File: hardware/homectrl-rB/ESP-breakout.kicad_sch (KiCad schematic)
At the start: 19 parts, among them J2 USB_C_Female_USB2_Small, SW1 SW_RESET, SW2 SW_BOOT, U1 ESP32-S3-WROOM-1

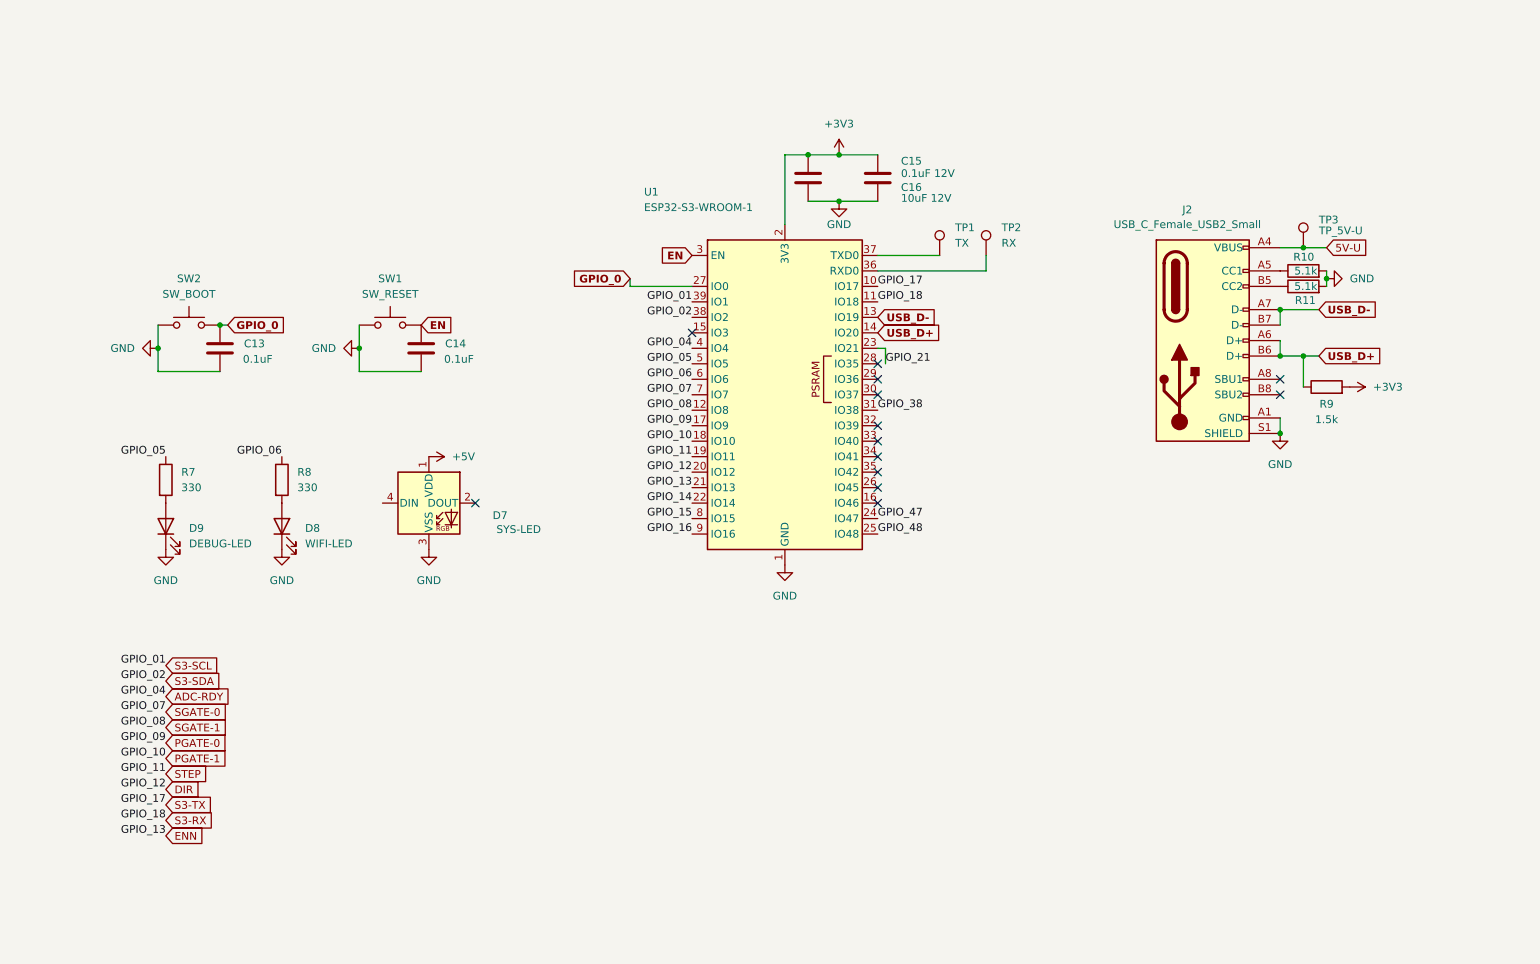
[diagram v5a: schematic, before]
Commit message: assign footprints
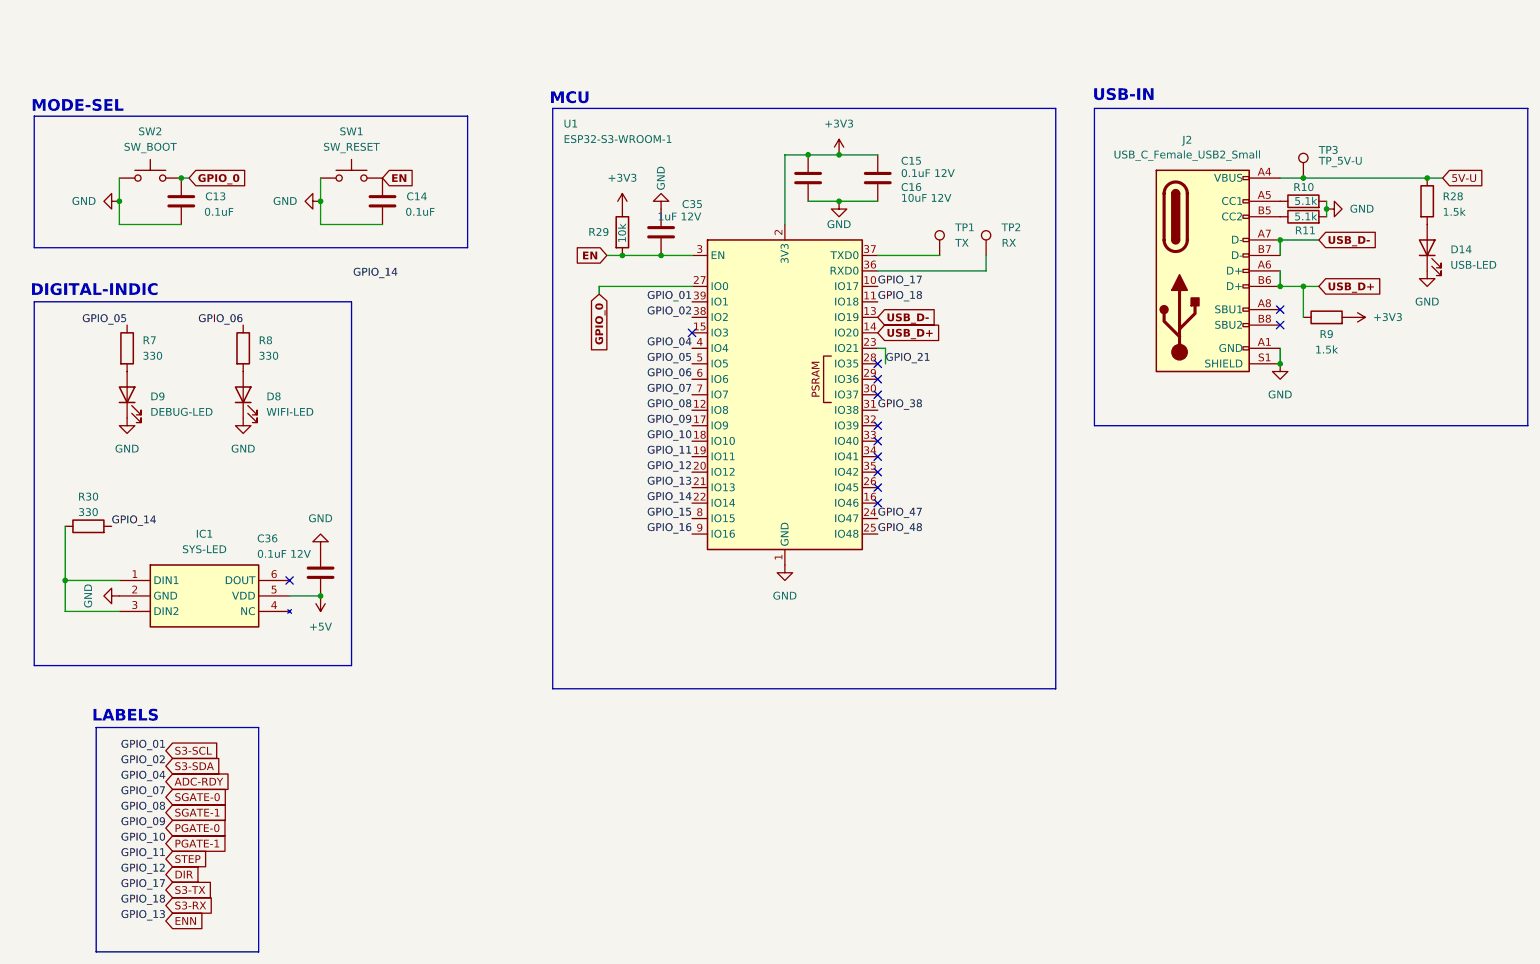
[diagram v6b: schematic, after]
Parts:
- removed D7: SYS-LED, LED_SMD:LED_WS2812B_PLCC4_5.0x5.0mm_P3.2mm, symbol LED:WS2812B
- added C35: 1uF 12V, Capacitor_SMD:C_0603_1608Metric, symbol Device:C
- added C36: 0.1uF 12V, Capacitor_SMD:C_0402_1005Metric, symbol Device:C
- added D14: USB-LED, LED_SMD:LED_0402_1005Metric, symbol Device:LED
- added IC1: SYS-LED, IN-PI20TBT5R5G5B:INPI20TBT5R5G5B, symbol IN-PI20TBT5R5G5B:IN-PI20TBT5R5G5B
- added R28: 1.5k, Resistor_SMD:R_0603_1608Metric, symbol Device:R
- added R29: 10k, Resistor_SMD:R_0402_1005Metric, symbol Device:R
- added R30: 330, Resistor_SMD:R_0402_1005Metric, symbol Device:R
- U1: footprint RF_Module:ESP32-S3-WROOM-1 -> ESP32-S3-WROOM-1-N16R2:XCVR_ESP32-S3-WROOM-1-N16R2
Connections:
- net +3V3: now also R29.1
- net +5V: now also C36.2, IC1.5 (VDD)
- net 5V-U: now also R28.1
- net EN: now also C35.1, R29.2
- net GND: now also C35.2, C36.1, D14.1 (K), IC1.2 (GND)
- net GPIO_14: now also R30.2
- new net: D14.2 (A), R28.2
- new net: IC1.1 (DIN1), IC1.3 (DIN2), R30.1
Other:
- note added: "DIGITAL-INDIC"
- note added: "LABELS"
- note added: "MCU"
- note added: "MODE-SEL"
- note added: "USB-IN"
- moved on the sheet: C13, C14, D8, D9, J2, R10, R11, R7, R8, R9, SW1, SW2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

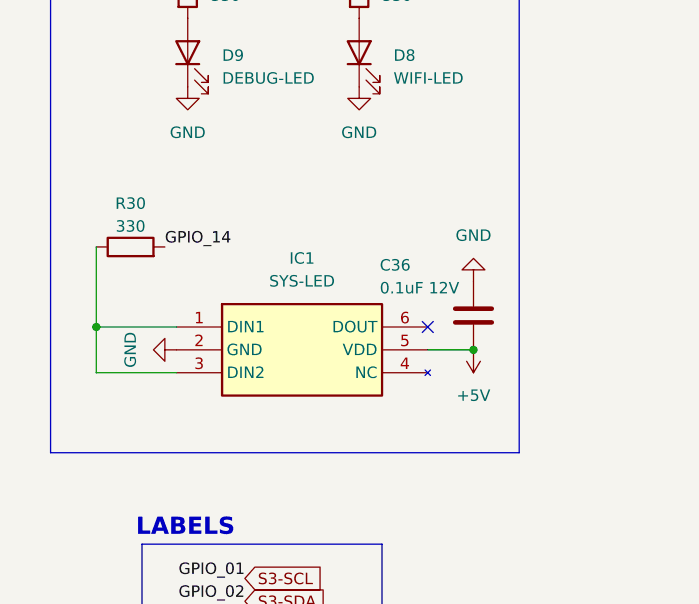
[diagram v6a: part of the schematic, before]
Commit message: layout work
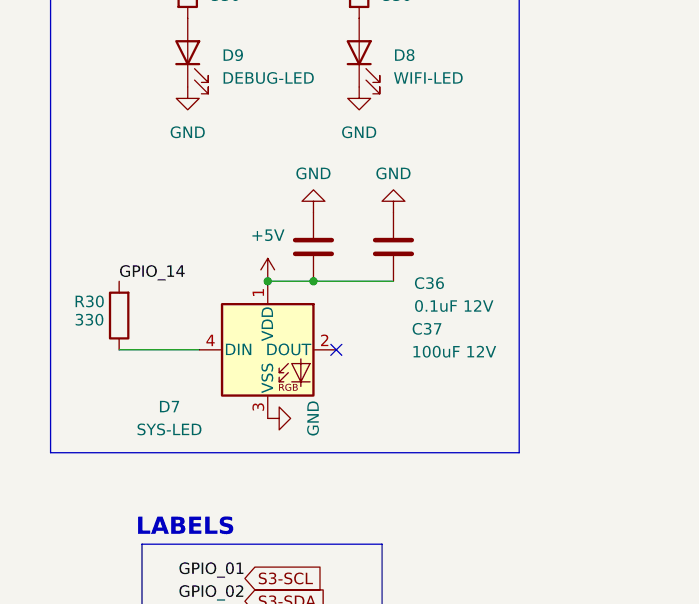
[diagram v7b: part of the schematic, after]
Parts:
- removed IC1: SYS-LED, IN-PI20TBT5R5G5B:INPI20TBT5R5G5B, symbol IN-PI20TBT5R5G5B:IN-PI20TBT5R5G5B
- added C37: 100uF 12V, Capacitor_SMD:C_1206_3216Metric, symbol Device:C
- added D7: SYS-LED, LED_SMD:LED_WS2812B_PLCC4_5.0x5.0mm_P3.2mm, symbol LED:WS2812B
- D14: footprint LED_SMD:LED_0402_1005Metric -> LED_SMD:LED_0603_1608Metric
- D8, D9: footprint Diode_SMD:D_0805_2012Metric -> LED_SMD:LED_0805_2012Metric
- R28: footprint Resistor_SMD:R_0603_1608Metric -> Resistor_SMD:R_0402_1005Metric
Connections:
- net +5V: now also C37.2, D7.1 (VDD)
- net GND: now also C37.1, D7.3 (VSS)
- net at R30.1: now also D7.4 (DIN)
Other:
- moved on the sheet: C36, R30

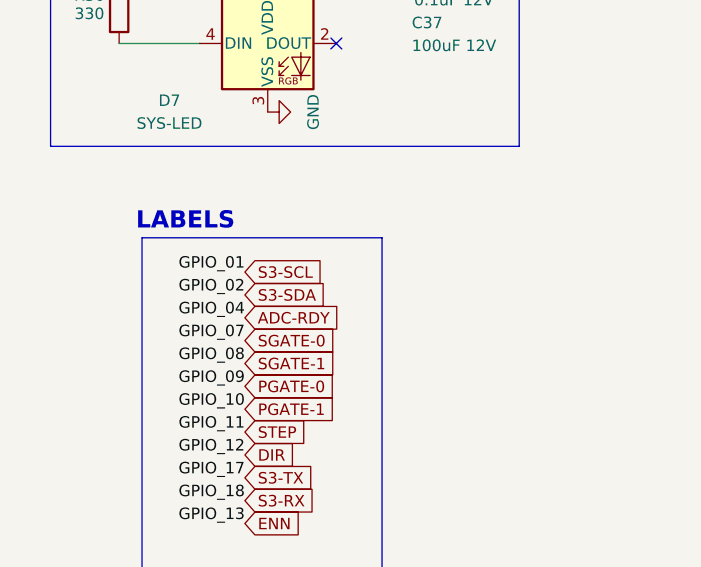
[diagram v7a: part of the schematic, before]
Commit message: routing work
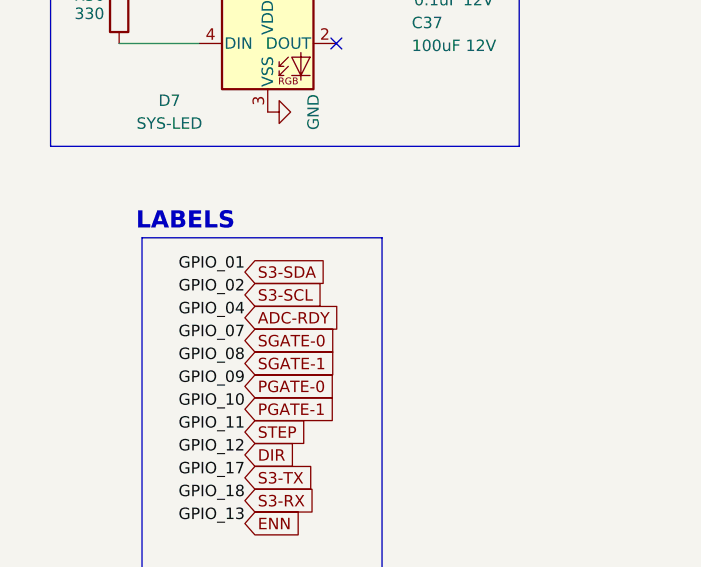
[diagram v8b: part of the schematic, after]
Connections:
- net S3-SCL: now also U1.38 (IO2); no longer U1.39 (IO1)
- net S3-SDA: now also U1.39 (IO1); no longer U1.38 (IO2)
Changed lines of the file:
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@@
+		)
+	)
+	(global_label "STEP"
+		(shape input)
+		(at 46.99 167.64 0)
+		(fields_autoplaced yes)
+		(effects
+			(font
+				(size 1.27 1.27)
+			)
+			(justify left)
+		)
+		(property "Intersheetrefs" "${INTERSHEET_REFS}"
+			(at 54.5713 167.64 0)
+			(effects
+				(font
+					(size 1.27 1.27)
+				)
+				(justify left)
+				(hide yes)
+			)
+		)
+	)
+	(global_label "ENN"
+		(shape input)
+		(at 46.99 177.8 0)
+		(fields_autoplaced yes)
+		(effects
+			(font
+				(size 1.27 1.27)
+			)
+			(justify left)
+		)
+		(property "Intersheetrefs" "${INTERSHEET_REFS}"
+			(at 53.7852 177.8 0)
+			(effects
+				(font
+					(size 1.27 1.27)
+				)
+				(justify left)
+				(hide yes)
+			)
+		)
+	)
+	(global_label "SGATE-1"
+		(shape input)
+		(at 46.99 160.02 0)
+		(fields_autoplaced yes)
+		(effects
+			(font
+				(size 1.27 1.27)
+			)
+			(justify left)
+		)
+		(property "Intersheetrefs" "${INTERSHEET_REFS}"
+			(at 58.4418 160.02 0)
+			(effects
+				(font
+					(size 1.27 1.27)
+				)
+				(justify left)
+				(hide yes)
+			)
+		)
+	)
+	(global_label "S3-SDA"
+		(shape input)
+		(at 46.99 149.86 0)
+		(fields_autoplaced yes)
+		(effects
+			(font
+				(size 1.27 1.27)
+			)
+			(justify left)
+		)
+		(property "Intersheetrefs" "${INTERSHEET_REFS}"
+			(at 57.5347 149.86 0)
+			(effects
+				(font
+					(size 1.27 1.27)
+				)
+				(justify left)
+				(hide yes)
+			)
 		)
 	)
 	(global_label "S3-SCL"
 		(shape input)
-		(at 46.99 149.86 0)
-		(fields_autoplaced yes)
-		(effects
-			(font
-				(size 1.27 1.27)
-			)
-			(justify left)
-		)
-		(property "Intersheetrefs" "${INTERSHEET_REFS}"
-			(at 57.4742 149.86 0)
-			(effects
-				(font
-					(size 1.27 1.27)
-				)
-				(justify left)
-				(hide yes)
-			)
-		)
-	)
-	(global_label "STEP"
-		(shape input)
-		(at 46.99 167.64 0)
-		(fields_autoplaced yes)
-		(effects
-			(font
-				(size 1.27 1.27)
-			)
-			(justify left)
-		)
-		(property "Intersheetrefs" "${INTERSHEET_REFS}"
-			(at 54.5713 167.64 0)
-			(effects
-				(font
-					(size 1.27 1.27)
-				)
-				(justify left)
-				(hide yes)
-			)
-		)
-	)
-	(global_label "ENN"
-		(shape input)
-		(at 46.99 177.8 0)
-		(fields_autoplaced yes)
-		(effects
-			(font
-				(size 1.27 1.27)
-			)
-			(justify left)
-		)
-		(property "Intersheetrefs" "${INTERSHEET_REFS}"
-			(at 53.7852 177.8 0)
-			(effects
-				(font
-					(size 1.27 1.27)
-				)
-				(justify left)
-				(hide yes)
-			)
-		)
-	)
-	(global_label "SGATE-1"
-		(shape input)
-		(at 46.99 160.02 0)
-		(fields_autoplaced yes)
-		(effects
-			(font
-				(size 1.27 1.27)
-			)
-			(justify left)
-		)
-		(property "Intersheetrefs" "${INTERSHEET_REFS}"
-			(at 58.4418 160.02 0)
+		(at 46.99 152.4 0)
+		(fields_autoplaced yes)
+		(effects
+			(font
+				(size 1.27 1.27)
+			)
+			(justify left)
+		)
+		(property "Intersheetrefs" "${INTERSHEET_REFS}"
+			(at 57.4742 152.4 0)
 			(effects
 				(font
@@
 			(effects
 				(font
-					(size 1.27 1.27)
-				)
-				(justify left)
-				(hide yes)
-			)
-		)
-	)
-	(global_label "S3-SDA"
-		(shape input)
-		(at 46.99 152.4 0)
-		(fields_autoplaced yes)
-		(effects
-			(font
-				(size 1.27 1.27)
-			)
-			(justify left)
-		)
-		(property "Intersheetrefs" "${INTERSHEET_REFS}"
-			(at 57.5347 152.4 0)
-			(effects
-				(font
